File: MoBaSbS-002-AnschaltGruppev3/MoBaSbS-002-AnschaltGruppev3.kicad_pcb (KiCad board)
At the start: 2 copper layers, 58.4 x 80 mm, 26 parts, among them IC1 TJA1057BT, IC2 SP3485EN-L_TR, J1 RJ45, J2 RJ45, P1 PSS254, P4 2x5_Buchse, P5 Wago, P6 Wago

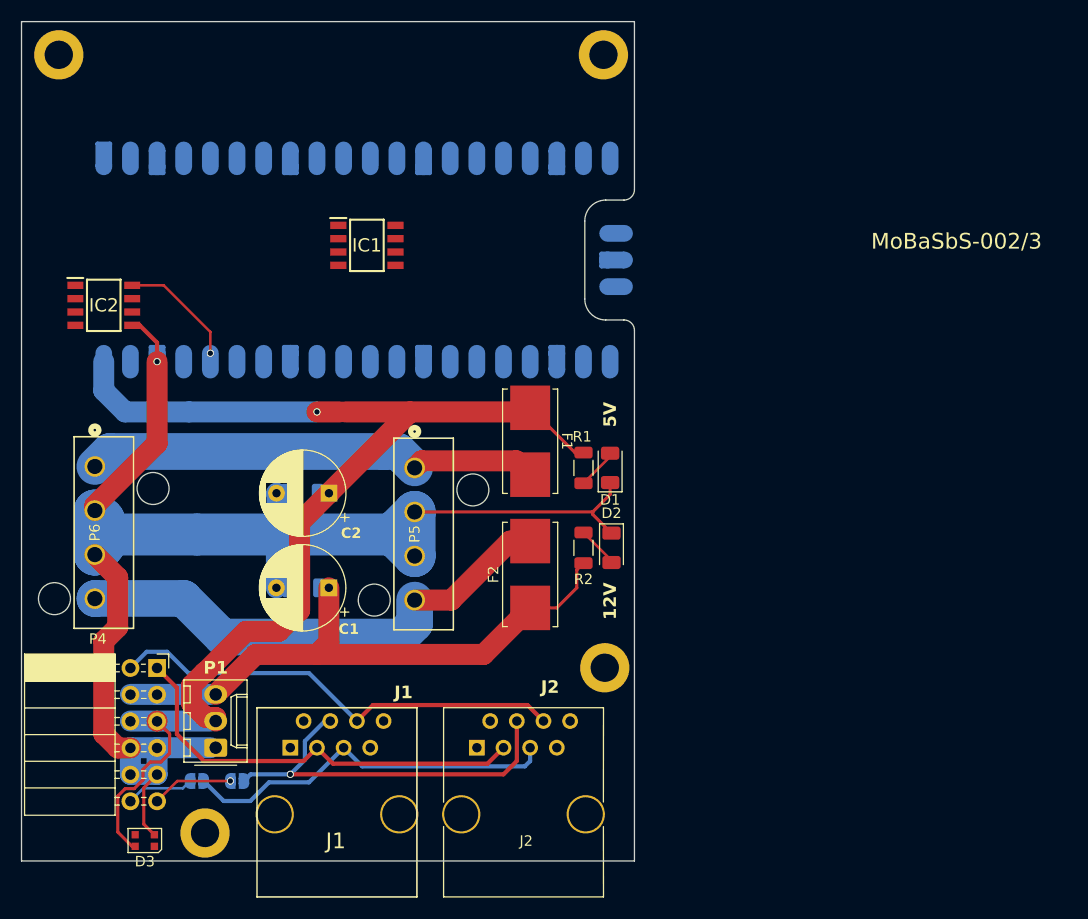
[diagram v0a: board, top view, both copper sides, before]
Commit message: Only some finishing touches left
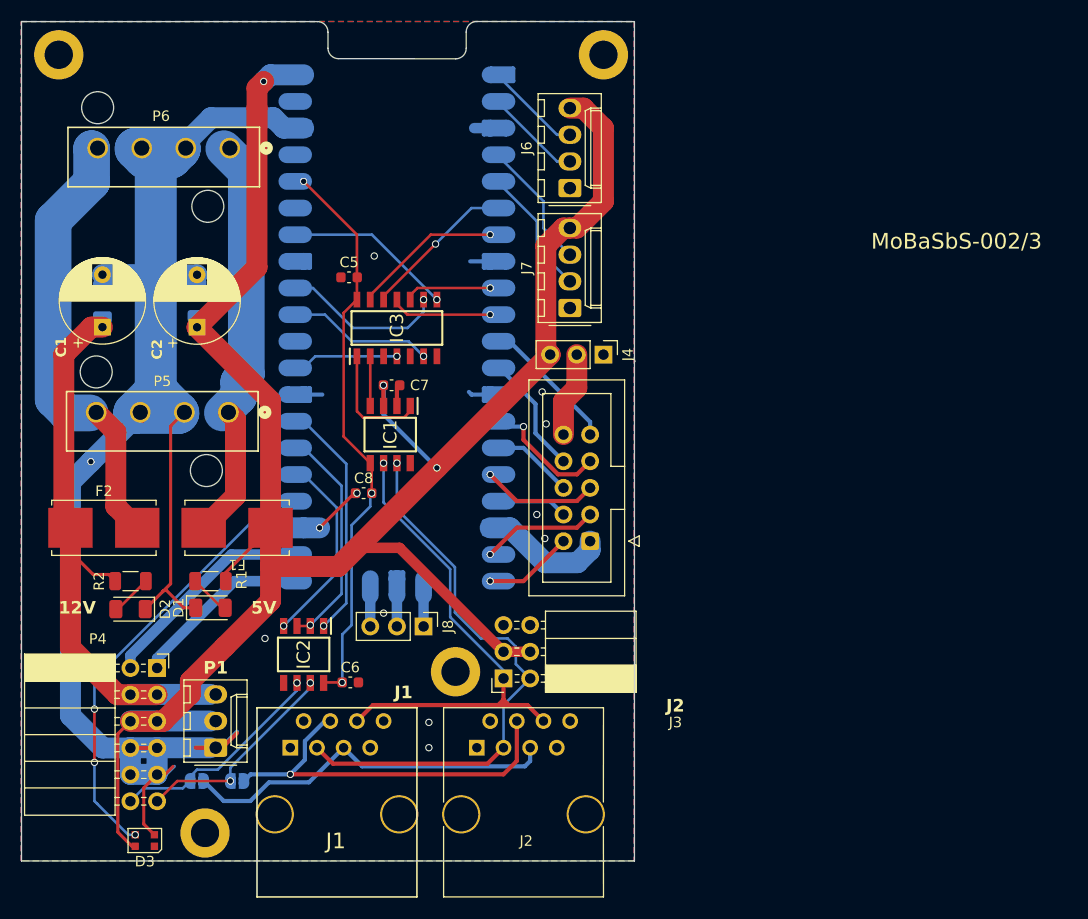
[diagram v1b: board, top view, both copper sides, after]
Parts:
- added C5: 100nF, Capacitor_SMD:C_0603_1608Metric, F.Cu at (139.2, 101.9)
- added C6: 100nF, Capacitor_SMD:C_0603_1608Metric, F.Cu at (139.3, 140.5)
- added C7: 100nF, Capacitor_SMD:C_0603_1608Metric, F.Cu at (143.2, 112.1)
- added C8: 100nF, Capacitor_SMD:C_0603_1608Metric, F.Cu at (140.6, 122.4)
- added IC3: MCP2518FDT-E_SL, CAN Controller:SOIC127P600X175-14N, F.Cu at (143.7, 106.7)
- added J3: Conn_02x03_Odd_Even, Connector_PinSocket_2.54mm:PinSocket_2x03_P2.54mm_Horizontal, F.Cu at (153.9, 140.1)
- added J4: Conn_01x03, Connector_PinHeader_2.54mm:PinHeader_1x03_P2.54mm_Vertical, F.Cu at (163.4, 109.2)
- added J5: Conn_02x05_Counter_Clockwise, Connector_IDC:IDC-Header_2x05_P2.54mm_Vertical, F.Cu at (162.1, 127.0)
- added J6: Conn_01x04, Connector_Molex:Molex_KK-254_AE-6410-04A_1x04_P2.54mm_Vertical, F.Cu at (160.2, 93.3)
- added J7: Conn_01x04, Connector_Molex:Molex_KK-254_AE-6410-04A_1x04_P2.54mm_Vertical, F.Cu at (160.2, 104.8)
- added J8: Conn_01x03, Connector_PinHeader_2.54mm:PinHeader_1x03_P2.54mm_Vertical, F.Cu at (146.3, 135.1)
- A1: footprint Module_RaspberryPi_Pico:RaspberryPi_Pico_Original_SMD -> Module_RaspberryPi_Pico:RaspberryPi_Pico_Original_SMD_HandSolder
- moved D2 46.2 mm to (118.3, 133.5), turned to 180 degrees
- moved R2 43.3 mm to (118.3, 130.8), turned to 180 degrees
- moved F2 40.9 mm to (115.8, 125.7), turned to 0 degrees
- moved D1 40.4 mm to (126.0, 133.3), turned to 0 degrees
- moved IC2 38.3 mm to (134.8, 137.8), turned to -90 degrees
- moved R1 37.2 mm to (126.0, 130.8), turned to 0 degrees
- moved C3 33.3 mm to (115.7, 104.2), turned to 90 degrees
- moved P6 33.0 mm to (127.8, 89.5), turned to 0 degrees
- moved C1 32.9 mm to (115.7, 106.6), turned to 90 degrees
- moved F1 29.1 mm to (128.5, 125.7), turned to 180 degrees
- moved C4 20.9 mm to (124.7, 104.1), turned to 90 degrees
- moved C2 20.2 mm to (124.7, 106.6), turned to 90 degrees
- moved P5 18.5 mm to (127.7, 114.7), turned to 0 degrees
- moved IC1 18.2 mm to (143.1, 116.8), turned to -90 degrees
- moved H4 14.2 mm to (149.3, 139.4)
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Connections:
- A1 pad 1: unconnected-(A1-GPIO0-Pad1) -> /IO_11
- A1 pad 10: unconnected-(A1-GPIO7-Pad10) -> /CAN_SDI
- A1 pad 11: unconnected-(A1-GPIO8-Pad11) -> /GPIO22
- A1 pad 12: unconnected-(A1-GPIO9-Pad12) -> /GPIO21
- A1 pad 14: unconnected-(A1-GPIO10-Pad14) -> /GPIO20
- A1 pad 15: unconnected-(A1-GPIO11-Pad15) -> /GPIO19
- A1 pad 16: unconnected-(A1-GPIO12-Pad16) -> /GPIO18
- A1 pad 17: unconnected-(A1-GPIO13-Pad17) -> /GPIO17
- A1 pad 19: unconnected-(A1-GPIO14-Pad19) -> /GPIO16
- A1 pad 2: unconnected-(A1-GPIO1-Pad2) -> /IO_12
- A1 pad 20: unconnected-(A1-GPIO15-Pad20) -> /GPIO15
- A1 pad 21: unconnected-(A1-GPIO16-Pad21) -> /I2C_SDA
- A1 pad 22: unconnected-(A1-GPIO17-Pad22) -> /I2C_SCL
- A1 pad 24: unconnected-(A1-GPIO18-Pad24) -> /WS2812
- A1 pad 25: unconnected-(A1-GPIO19-Pad25) -> /MOBA_OUT
- A1 pad 26: unconnected-(A1-GPIO20-Pad26) -> /MOBA_WRITE
- A1 pad 27: unconnected-(A1-GPIO21-Pad27) -> /MOBA_IN
- A1 pad 29: unconnected-(A1-GPIO22-Pad29) -> /CAN_INT
- A1 pad 31: unconnected-(A1-GPIO26_ADC0-Pad31) -> /CAN_OSC
- A1 pad 32: unconnected-(A1-GPIO27_ADC1-Pad32) -> /CAN_INT0
- A1 pad 34: unconnected-(A1-GPIO28_ADC2-Pad34) -> /CAN_INT1
- A1 pad 4: unconnected-(A1-GPIO2-Pad4) -> /IO_21
- A1 pad 5: unconnected-(A1-GPIO3-Pad5) -> /IO_22
- A1 pad 6: unconnected-(A1-GPIO4-Pad6) -> /CAN_SDO
- A1 pad 7: unconnected-(A1-GPIO5-Pad7) -> /CAN_CS
- A1 pad 9: unconnected-(A1-GPIO6-Pad9) -> /CAN_SCK
- A1 pad D1: (no net) -> /SWDCLK
- A1 pad D2: (no net) -> GND
- A1 pad D3: (no net) -> /SWDIO
- D3 pad 3: unconnected-(D3-DIN-Pad3) -> /WS2812
- IC1 pad 1: unconnected-(IC1-TXD-Pad1) -> /CAN_TX
- IC1 pad 2: unconnected-(IC1-GND-Pad2) -> GND
- IC1 pad 3: unconnected-(IC1-VCC-Pad3) -> +5V
- IC1 pad 4: unconnected-(IC1-RXD-Pad4) -> /CAN_RX
- IC1 pad 5: unconnected-(IC1-VIO-Pad5) -> /+3V3
- IC1 pad 6: unconnected-(IC1-CANL-Pad6) -> /CAN_H
- IC1 pad 7: unconnected-(IC1-CANH-Pad7) -> /CAN_L
- IC2 pad 1: unconnected-(IC2-RO-Pad1) -> /MOBA_IN
- IC2 pad 2: unconnected-(IC2-~{RE}-Pad2) -> /MOBA_WRITE
- IC2 pad 3: unconnected-(IC2-DE-Pad3) -> /MOBA_WRITE
- IC2 pad 4: unconnected-(IC2-DI-Pad4) -> /MOBA_OUT
- J1 pad 3: Net-(J1-Pin_3) -> /CAN_L
- J1 pad 4: Net-(IC2-B) -> Net-(J1-Pin_4)
- J1 pad 5: Net-(IC2-A) -> Net-(J1-Pin_5)
- J1 pad 6: Net-(J1-Pin_6) -> /CAN_H
- J2 pad 3: Net-(J1-Pin_3) -> /CAN_L
- J2 pad 4: Net-(IC2-B) -> Net-(J1-Pin_4)
- J2 pad 5: Net-(IC2-A) -> Net-(J1-Pin_5)
- J2 pad 6: Net-(J1-Pin_6) -> /CAN_H
- JP1 pad 1: Net-(JP1-A) -> Net-(IC2-B)
- JP1 pad 2: Net-(IC2-B) -> Net-(J1-Pin_4)
- JP2 pad 1: Net-(JP2-A) -> Net-(IC2-A)
- JP2 pad 2: Net-(IC2-A) -> Net-(J1-Pin_5)
- P4 pad 1: Net-(J1-Pin_3) -> /I2C_SDA
- P4 pad 11: Net-(JP1-A) -> Net-(IC2-B)
- P4 pad 12: Net-(JP2-A) -> Net-(IC2-A)
- P4 pad 2: Net-(J1-Pin_6) -> /I2C_SCL
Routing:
- net +5V: track 116.2 -> 203.0 mm, vias 1 -> 3
- net GND: track 144.9 -> 201.3 mm, vias 1 -> 12
- net /CAN_L: track 0.00 -> 54.3 mm, vias 0 -> 1
- net /CAN_H: track 0.00 -> 49.5 mm, vias 0 -> 1
- net Net-(J1-Pin_6): track 44.0 -> 0.00 mm
- net /WS2812: track 0.00 -> 43.8 mm, vias 0 -> 3
- net /+3V3: track 11.3 -> 54.4 mm, vias 1 -> 3
- net Net-(J1-Pin_3): track 41.4 -> 0.00 mm
- net Net-(J1-Pin_4): track 0.00 -> 37.6 mm, vias 0 -> 1
- net Net-(J1-Pin_5): track 0.00 -> 36.2 mm
- net /MOBA_IN: track 0.00 -> 22.1 mm, vias 0 -> 1
- net /I2C_SCL: track 0.00 -> 21.7 mm
- net /MOBA_WRITE: track 0.00 -> 21.4 mm, vias 0 -> 1
- net /MOBA_OUT: track 0.00 -> 18.3 mm, vias 0 -> 1
- net /I2C_SDA: track 0.00 -> 17.9 mm
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- added copper zone on B.Cu, net GND
- added copper zone on F.Cu, net GND
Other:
- outline, holes or cut-outs redrawn
